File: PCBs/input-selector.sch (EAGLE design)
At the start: 30 parts, among them IC1 MCP23S17SO, IC2 ULN2803, IC3 ULN2803, K1 AGQ2104H, K2 AGQ2104H, K3 AGQ2104H

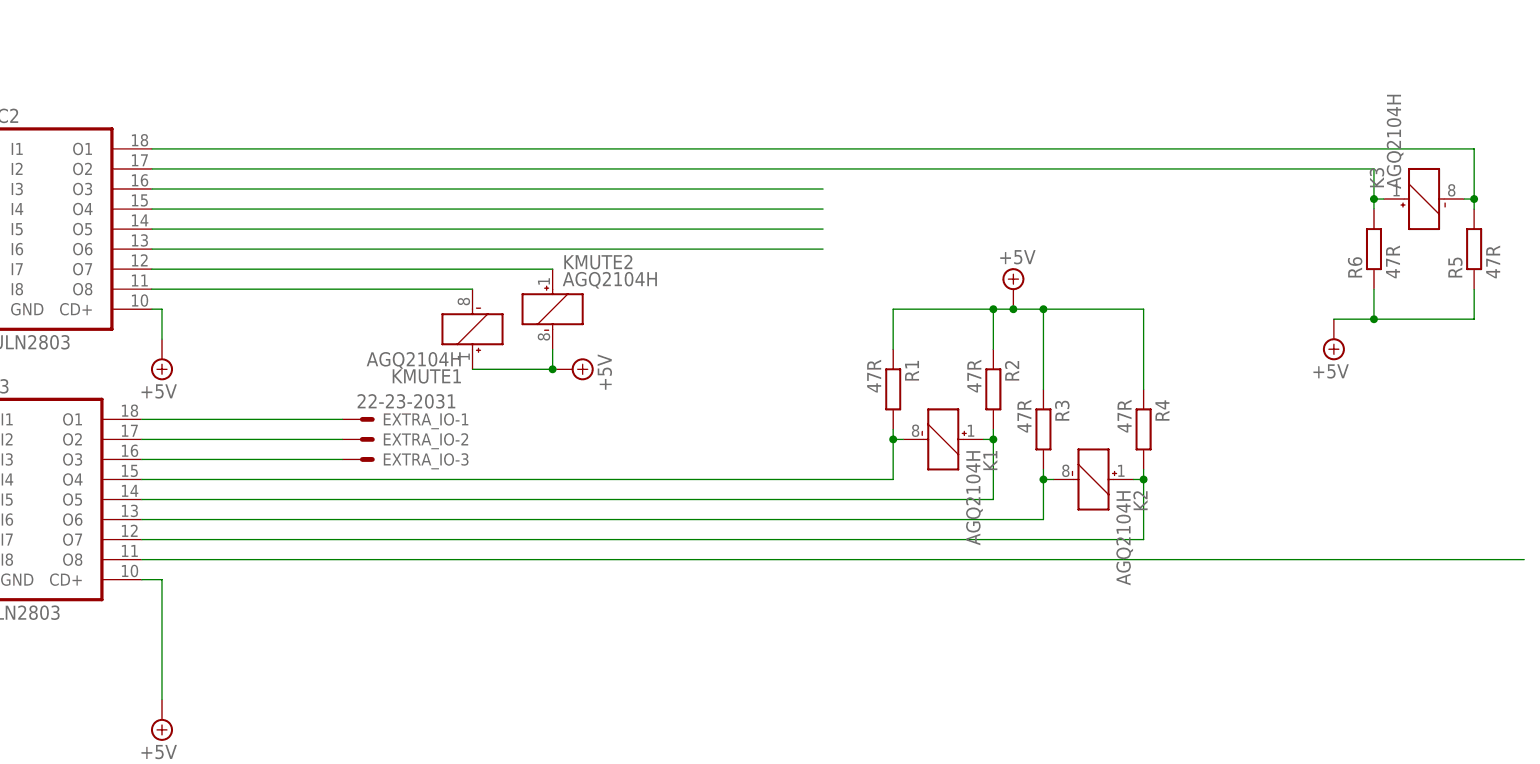
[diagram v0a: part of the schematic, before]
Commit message: Finished up connections
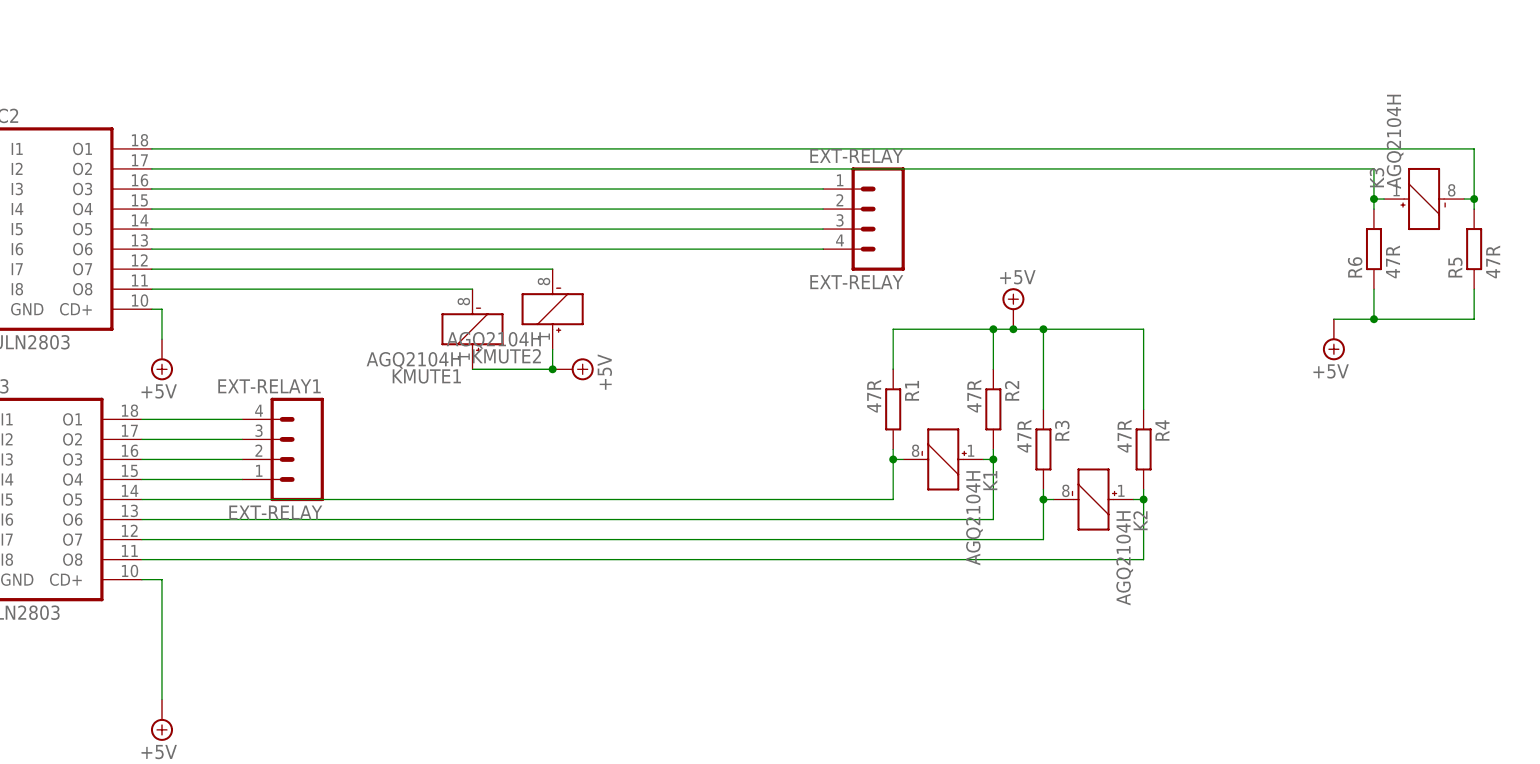
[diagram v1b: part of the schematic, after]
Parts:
- removed EXTRA_IO: 22-23-2031, con-molex:22-23-2031
- added EXT-RELAY, EXT-RELAY1: EXT-RELAY, SparkFun-Connectors:M04POLAR
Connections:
- net +5V: now also KMUTE2G$1.+; no longer KMUTE2G$1.-
- net N$10: now also EXT-RELAY1.3, IC3.O2; no longer EXTRA_IO-1.S, IC3.O1
- net N$11: now also EXT-RELAY.1
- net N$12: now also IC3.O8; no longer IC3.O7
- net N$13: now also EXT-RELAY1.4, IC3.O1; no longer IC3.O8
- net N$15: now also EXT-RELAY.2
- net N$16: now also EXT-RELAY.4
- net N$19: now also KMUTE2G$1.-; no longer KMUTE2G$1.+
- net N$2: now also EXT-RELAY1.1, IC3.O4; no longer EXTRA_IO-2.S, IC3.O2
- net N$23: now also EXT-RELAY.3
- net N$4: now also EXT-RELAY1.2; no longer EXTRA_IO-3.S
- net N$5: now also IC3.O5; no longer IC3.O4
- net N$8: now also IC3.O6; no longer IC3.O5
- net N$9: now also IC3.O7; no longer IC3.O6
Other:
- moved on the sheet: K1, K2, KMUTE2, R1, R2, R3, R4
